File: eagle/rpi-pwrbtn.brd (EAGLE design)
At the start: 63.5 x 63.5 mm, 16 parts, among them IC1 ATTINY85-20SU, IC2 +3V3, X1 ALTPWR

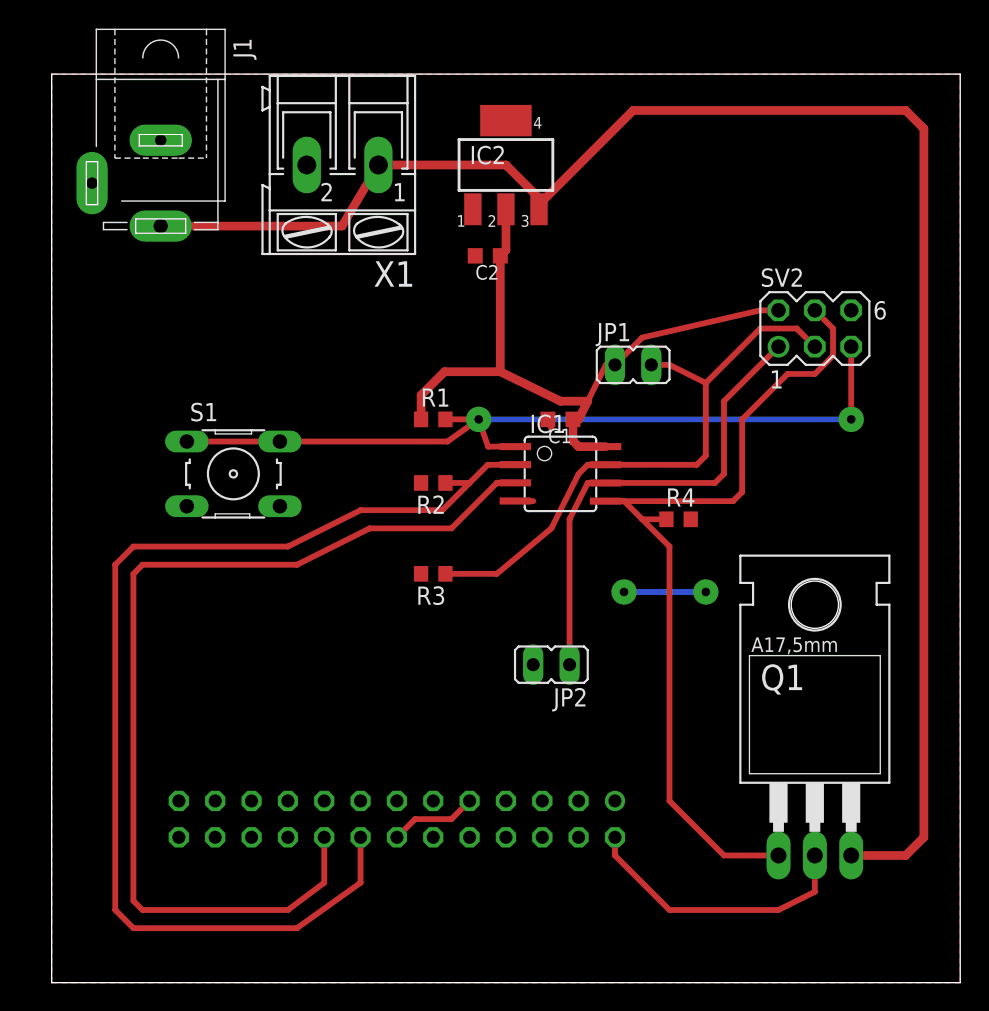
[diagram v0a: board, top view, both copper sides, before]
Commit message: Update through-hole schematic and board files.
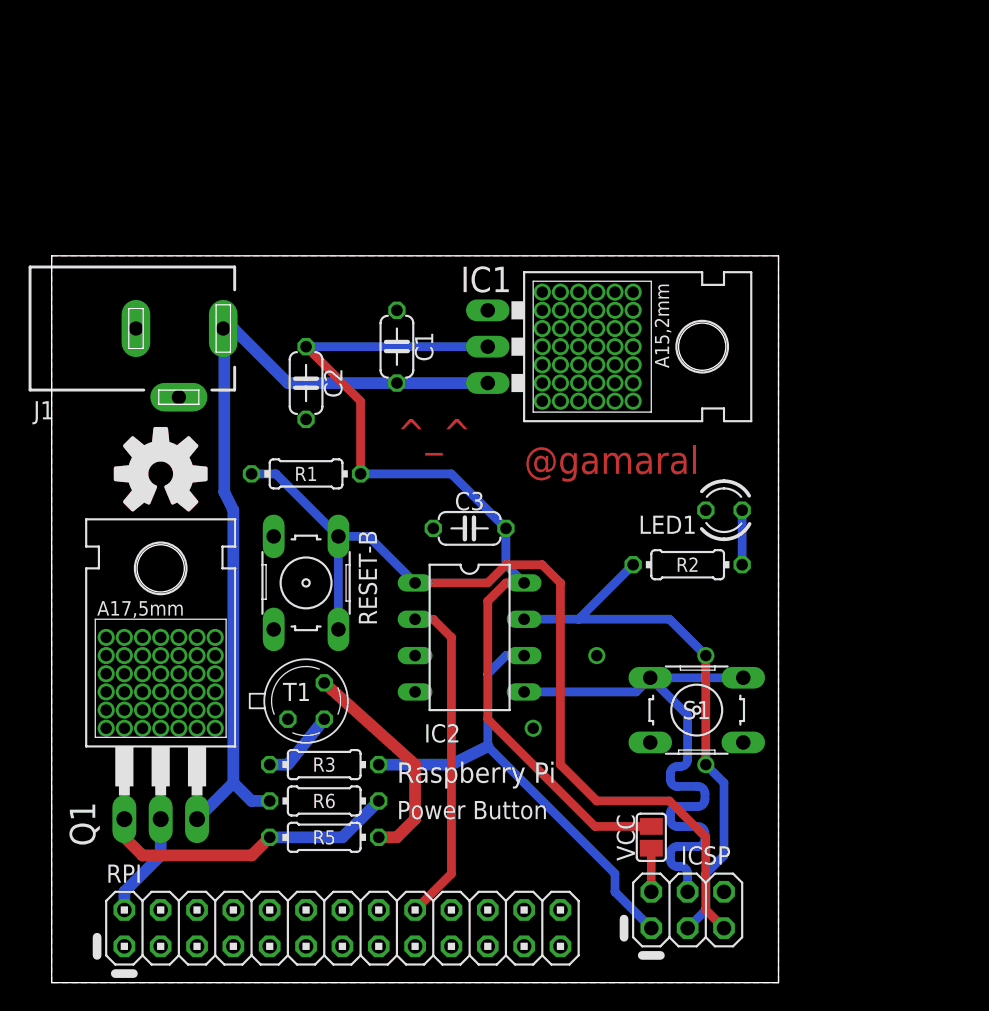
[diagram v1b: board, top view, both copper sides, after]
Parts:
- removed JP1: BTN, jumper:JP1
- removed JP2: LED, jumper:JP1
- removed R4: 10k, resistor:R0603
- removed SV1: RPI, con-lsta:FE13-2
- removed SV2: ICSP, con-lstb:MA03-2
- removed X1: ALTPWR, con-ptr500:AK300/2
- added C3: 100nF, resistor:C050-024X044
- added ICSP: (no value), pinhead:2X03
- added LED1: STATUS, led:LED3MM
- added R5: 6k2, resistor:0204/7
- added R6: 62k, resistor:0204/7
- added RESET-B: RESET, switch-omron:B3F-10XX
- added RPI: (no value), pinhead:2X13
- added T1: 2N2222, transistor:TO18
- added VCC: (no value), jumper:SJ
- C1: value 0.1µF -> 100nF; device resistor:C0603K -> resistor:C050-024X044
- C2: device resistor:C0603K -> resistor:C050-024X044
- IC1: value ATTINY85-20SU -> LD117AV33; device gamaral:SOIC8 -> v-reg:TO220L1
- IC2: value +3V3 -> TINY85P; device linear:SOT223 -> gamaral:DIL08
- J1: device con-jack:SPC4078 -> con-jack:DCJ0303
- Q1: value (none) -> TIP125; device transistor-power:TO220BH -> transistor-power:TO220AH
- R1: device resistor:R0603 -> resistor:0204/7
- R2: value 10k -> 330R; device resistor:R0603 -> resistor:0204/7
- R3: value 10k -> 240k; device resistor:R0603 -> resistor:0204/7
- S1: value (none) -> PWR
- moved Q1 45.8 mm to (7.62, 17.8)
- moved S1 36.4 mm to (45.1, 19.1), turned to 180 degrees
- moved IC2 33.1 mm to (29.2, 24.1), turned to 270 degrees
- moved R2 18.7 mm to (44.5, 29.2), turned to 0 degrees
- moved C2 15.5 mm to (17.8, 41.9), turned to 270 degrees
- moved R3 15.4 mm to (19.1, 15.2)
- moved C1 12.5 mm to (24.1, 44.5), turned to 90 degrees
- moved J1 10.2 mm to (8.89, 45.7)
- moved R1 9.67 mm to (17.8, 35.6), turned to 180 degrees
- moved IC1 8.98 mm to (34.3, 44.5)
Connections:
- removed net BTN: IC1.7, JP1.2, R3.1, SV2.3
- removed net LED: IC1.6, JP2.1, SV2.1
- removed net PWR: IC1.5, Q1.G, R4.1, SV2.4
- removed net READY: IC1.2, R2.1, SV1.16
- removed net SHUTDOWN: IC1.3, SV1.18
- new net ICSP-VCC: ICSP.2, VCC.1
- new net N$1: LED1.A, R2.2
- new net N$3: Q1.C, RPI.2
- new net N$4: Q1.B, R5.2, R6.1
- new net N$5: R3.2, T1.2
- new net N$6: R5.1, T1.3
- new net RPI-IO: IC2.2, RPI.18
- new net RPI-LED: IC2.7, ICSP.3, R2.1
- new net RPI-USR: IC2.5, ICSP.4, S1.3, S1.4
- net +3V3: now also C3.1, IC1.2, IC2.8, VCC.2; no longer C1.1, IC1.8, IC2.2, JP1.1, SV2.2
- net +5V: now also C1.1, IC1.3, J1.1, Q1.E, R6.2; no longer IC2.3, J1.3, Q1.S, X1.1
- net GND: now also C3.2, IC1.1, IC2.4, ICSP.6, J1.2, J1.3, LED1.K, RESET-B.3, RESET-B.4, RPI.14, RPI.20, RPI.25, RPI.6, RPI.9, S1.1, S1.2, T1.1; no longer IC1.4, IC2.1, J1.1, JP2.2, R2.2, R3.2, R4.2, S1.3, S1.4, SV1.14, SV1.20, SV1.25, SV1.6, SV1.9, SV2.6, X1.2
- net RESET: now also IC2.1, ICSP.5, RESET-B.1, RESET-B.2; no longer IC1.1, S1.1, S1.2, SV2.5
- net RPI-PWR: now also IC2.6, ICSP.1, R3.1; no longer Q1.D, SV1.2
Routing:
- net READY: track 78.1 -> 0.00 mm
- net SHUTDOWN: track 69.1 -> 0.00 mm
- net PWR: track 61.2 -> 0.00 mm
- net +5V: track 115.6 -> 58.6 mm
- net BTN: track 41.1 -> 0.00 mm
- net RPI-USR: track 0.00 -> 40.4 mm
- net RPI-LED: track 0.00 -> 39.8 mm, vias 0 -> 2
- net LED: track 33.3 -> 0.00 mm
- net N$2: track 0.00 -> 30.0 mm
- net RPI-IO: track 0.00 -> 23.2 mm
- net N$4: track 0.00 -> 21.2 mm
- net +3V3: track 47.7 -> 65.1 mm
- net N$6: track 0.00 -> 15.4 mm
- net RPI-PWR: track 19.7 -> 33.5 mm
- net GND: track 13.8 -> 0.00 mm, vias 2 -> 86
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- added copper zone on layer 16, net GND
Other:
- board size 63.5 x 63.5 mm -> 50.8 x 50.8 mm
- board text added: "@gamaral"
- board text added: "Power Button"
- board text added: "REV 01-TL"
- board text added: "Raspberry Pi"
- board text added: "^_^"
